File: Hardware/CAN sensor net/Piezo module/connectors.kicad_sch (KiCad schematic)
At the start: 8 parts, among them J1 532610671, J2 532610671, J3 USB_B_Micro, J4 530470310, U7 USBLC6-2SC6

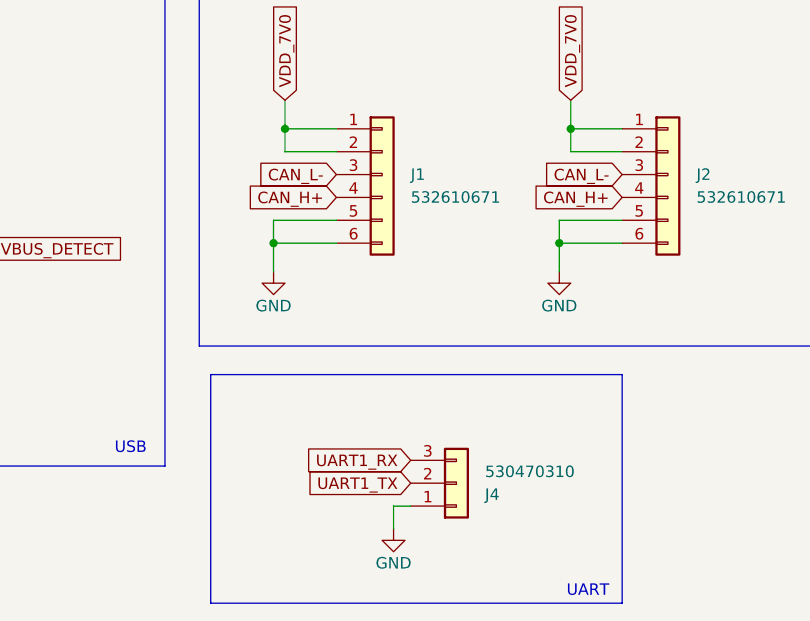
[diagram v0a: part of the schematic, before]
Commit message: Piezo concept (full)
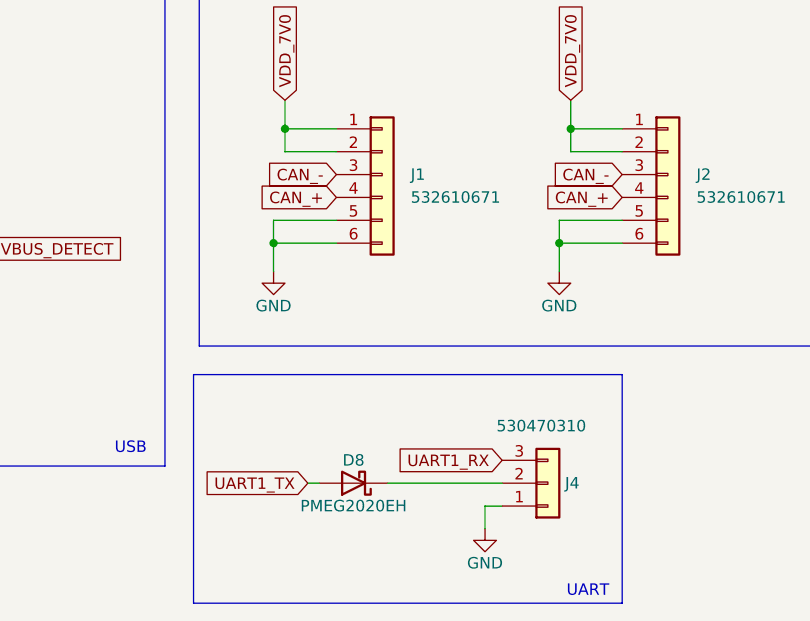
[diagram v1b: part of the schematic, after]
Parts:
- added D8: PMEG2020EH, Diode_SMD:D_SOD-123F, symbol Device:D_Schottky
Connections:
- net UART1_TX: now also D8.2 (A); no longer J4.2 (Pin_2)
- net CAN_H+ renamed CAN_+
- net CAN_L- renamed CAN_-
- new net: D8.1 (K), J4.2 (Pin_2)
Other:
- moved on the sheet: J4
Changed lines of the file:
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@@
 	(wire
 		(pts
+			(xy 174.625 79.375) (xy 175.895 79.375)
+		)
+		(stroke
+			(width 0)
+			(type default)
+		)
+	)
+	(wire
+		(pts
 			(xy 131.445 53.34) (xy 131.445 54.61)
 		)
@@
 	(wire
 		(pts
-			(xy 186.055 81.915) (xy 184.15 81.915)
+			(xy 196.215 81.915) (xy 194.31 81.915)
 		)
 		(stroke
@@
 	(wire
 		(pts
-			(xy 184.15 81.915) (xy 184.15 84.455)
+			(xy 194.31 81.915) (xy 194.31 84.455)
 		)
 		(stroke
@@
 	(wire
 		(pts
+			(xy 196.215 79.375) (xy 183.515 79.375)
+		)
+		(stroke
+			(width 0)
+			(type default)
+		)
+	)
+	(wire
+		(pts
 			(xy 97.155 64.77) (xy 97.155 66.675)
 		)
@@
 	(polyline
 		(pts
-			(xy 163.83 92.71) (xy 163.83 67.31)
+			(xy 161.925 92.71) (xy 161.925 67.31)
 		)
 		(stroke
@@
 	(polyline
 		(pts
-			(xy 163.83 92.71) (xy 209.55 92.71)
+			(xy 161.925 92.71) (xy 209.55 92.71)
 		)
 		(stroke
@@
 	(polyline
 		(pts
-			(xy 163.83 67.31) (xy 209.55 67.31)
+			(xy 161.925 67.31) (xy 209.55 67.31)
 		)
 		(stroke
@@
 		)
 	)
-	(global_label "CAN_L-"
+	(global_label "CAN_-"
 		(shape input)
 		(at 209.55 45.085 180)
@@
 		)
 		(property "Intersheetrefs" "${INTERSHEET_REFS}"
-			(at 199.3076 45.085 0)
+			(at 200.3357 45.085 0)
 			(effects
 				(font
@@
 	(global_label "UART1_TX"
 		(shape input)
-		(at 186.055 79.375 180)
+		(at 174.625 79.375 180)
 		(fields_autoplaced yes)
 		(effects
@@
 		)
 		(property "Intersheetrefs" "${INTERSHEET_REFS}"
-			(at 174.0589 79.375 0)
+			(at 162.6289 79.375 0)
 			(effects
 				(font
@@
 		)
 	)
-	(global_label "CAN_H+"
+	(global_label "CAN_+"
 		(shape input)
 		(at 209.55 47.625 180)
@@
 		)
 		(property "Intersheetrefs" "${INTERSHEET_REFS}"
-			(at 199.0052 47.625 0)
+			(at 200.3357 47.625 0)
 			(effects
 				(font
@@
 		)
 	)
-	(global_label "CAN_H+"
+	(global_label "CAN_+"
 		(shape input)
 		(at 177.8 47.625 180)
@@
 		)
 		(property "Intersheetrefs" "${INTERSHEET_REFS}"
-			(at 167.2552 47.625 0)
+			(at 168.5857 47.625 0)
 			(effects
 				(font
@@
 	(global_label "UART1_RX"
 		(shape input)
-		(at 186.055 76.835 180)
+		(at 196.215 76.835 180)
 		(fields_autoplaced yes)
 		(effects
@@
 		)
 		(property "Intersheetrefs" "${INTERSHEET_REFS}"
-			(at 173.7565 76.835 0)
+			(at 183.9165 76.835 0)
 			(effects
 				(font
@@
 		)
 	)
-	(global_label "CAN_L-"
+	(global_label "CAN_-"
 		(shape input)
 		(at 177.8 45.085 180)
@@
 		)
 		(property "Intersheetrefs" "${INTERSHEET_REFS}"
-			(at 167.5576 45.085 0)
+			(at 168.5857 45.085 0)
 			(effects
 				(font
@@
 		(pin "1"
 		)
+		(pin "MP"
+		)
 		(instances
 			(project "Piezo module"
@@
 	)
 	(symbol
+		(lib_id "Device:D_Schottky")
+		(at 179.705 79.375 180)
+		(unit 1)
+		(exclude_from_sim no)
+		(in_bom yes)
+		(on_board yes)
+		(dnp no)
+		(property "Reference" "D8"
+			(at 179.705 76.835 0)
+			(effects
+				(font
+					(size 1.27 1.27)
+				)
+			)
+		)
+		(property "Value" "PMEG2020EH"
+			(at 179.705 81.915 0)
+			(effects
+				(font
+					(size 1.27 1.27)
+				)
+			)
+		)
+		(property "Footprint" "Diode_SMD:D_SOD-123F"
+			(at 179.705 79.375 0)
+			(effects
+				(font
+					(size 1.27 1.27)
+				)
+				(hide yes)
+			)
+		)
+		(property "Datasheet" "~"
+			(at 179.705 79.375 0)
+			(effects
+				(font
+					(size 1.27 1.27)
+				)
+				(hide yes)
+			)
+		)
+		(property "Description" "Schottky diode"
+			(at 179.705 79.375 0)
+			(effects
+				(font
+					(size 1.27 1.27)
+				)
+				(hide yes)
+			)
+		)
+		(pin "2"
+		)
+		(pin "1"
+		)
+		(instances
+			(project "Piezo module"
+				(path "/0a58466e-2312-402a-82c7-7de62fe91dff/33325e08-e21c-439d-a7db-dde9f8ca3ce6"
+					(reference "D8")
+					(unit 1)
+				)
+			)
+		)
+	)
+	(symbol
 		(lib_name "GND_1")
 		(lib_id "power:GND")
@@
 		(lib_name "GND_1")
 		(lib_id "power:GND")
-		(at 184.15 84.455 0)
+		(at 194.31 84.455 0)
 		(unit 1)
 		(exclude_from_sim no)
@@
 		(dnp no)
 		(property "Reference" "#PWR018"
-			(at 184.15 90.805 0)
+			(at 194.31 90.805 0)
 			(effects
 				(font
@@
 		)
 		(property "Value" "GND"
-			(at 184.15 88.265 0)
+			(at 194.31 88.265 0)
 			(effects
 				(font
@@
 		)
 		(property "Footprint" ""
-			(at 184.15 84.455 0)
+			(at 194.31 84.455 0)
 			(effects
 				(font
@@
 		)
 		(property "Datasheet" ""
-			(at 184.15 84.455 0)
+			(at 194.31 84.455 0)
 			(effects
 				(font
@@
 		)
 		(property "Description" "Power symbol creates a global label with name \"GND\" , ground"
-			(at 184.15 84.455 0)
+			(at 194.31 84.455 0)
 			(effects
 				(font
@@
 	)
 	(symbol
+		(lib_name "Conn_01x06_1")
 		(lib_id "Connector_Generic:Conn_01x06")
 		(at 182.88 45.085 0)
@@
 		(pin "1"
 		)
+		(pin "MP"
+		)
 		(instances
 			(project "Piezo module"
@@
 	(symbol
 		(lib_id "Connector_Generic:Conn_01x03")
-		(at 191.135 79.375 0)
+		(at 201.295 79.375 0)
 		(mirror x)
 		(unit 1)
@@
 		(dnp no)
 		(property "Reference" "J4"
-			(at 194.31 80.6451 0)
+			(at 203.2 79.375 0)
 			(effects
 				(font
@@
 		)
 		(property "Value" "530470310"
-			(at 194.31 78.1051 0)
+			(at 195.58 73.025 0)
 			(effects
 				(font
@@
 		)
 		(property "Footprint" "Connector_Molex:Molex_PicoBlade_53261-0371_1x03-1MP_P1.25mm_Horizontal"
-			(at 191.135 79.375 0)
+			(at 201.295 79.375 0)
 			(effects
 				(font
@@
 		)
 		(property "Datasheet" "~"
-			(at 191.135 79.375 0)
+			(at 201.295 79.375 0)
 			(effects
 				(font
@@
 		)
 		(property "Description" "Generic connector, single row, 01x03, script generated (kicad-library-utils/schlib/autogen/connector/)"
-			(at 191.135 79.375 0)
+			(at 201.295 79.375 0)
 			(effects
 				(font
@@
 		(pin "1"
 		)
+		(pin "MP"
+		)
 		(instances

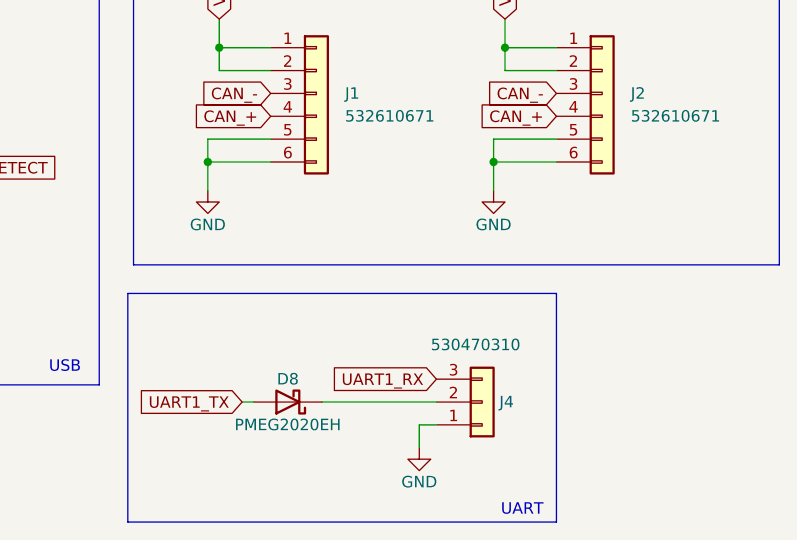
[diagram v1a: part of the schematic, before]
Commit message: Piezo production
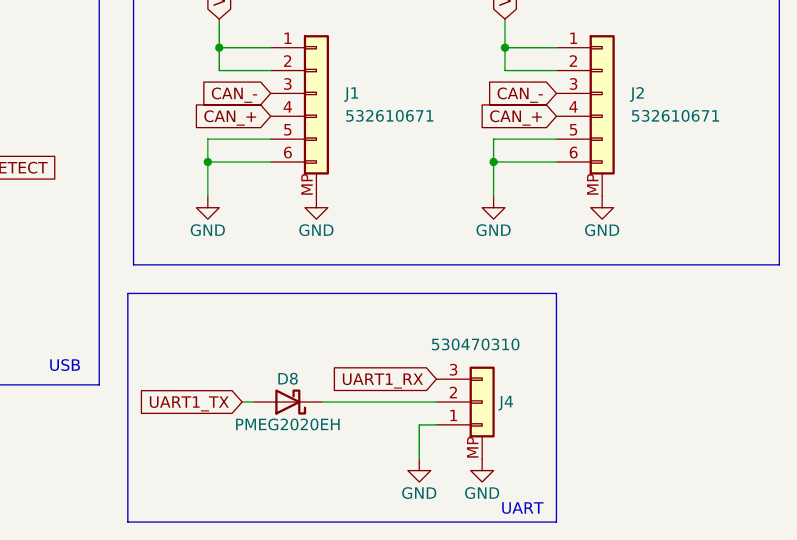
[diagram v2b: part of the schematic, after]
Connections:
- net GND: now also J1.MP, J2.MP, J4.MP
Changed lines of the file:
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@@
 	(wire
 		(pts
-			(xy 202.565 55.88) (xy 202.565 52.705)
+			(xy 202.565 56.515) (xy 202.565 52.705)
 		)
 		(stroke
@@
 	(wire
 		(pts
-			(xy 194.31 81.915) (xy 194.31 84.455)
+			(xy 194.31 81.915) (xy 194.31 85.725)
 		)
 		(stroke
@@
 	(wire
 		(pts
-			(xy 170.815 55.88) (xy 170.815 52.705)
+			(xy 170.815 56.515) (xy 170.815 52.705)
 		)
 		(stroke
@@
 	(symbol
 		(lib_id "power:GND")
+		(at 214.63 56.515 0)
+		(unit 1)
+		(exclude_from_sim no)
+		(in_bom yes)
+		(on_board yes)
+		(dnp no)
+		(property "Reference" "#PWR026"
+			(at 214.63 62.865 0)
+			(effects
+				(font
+					(size 1.27 1.27)
+				)
+				(hide yes)
+			)
+		)
+		(property "Value" "GND"
+			(at 214.63 60.325 0)
+			(effects
+				(font
+					(size 1.27 1.27)
+				)
+			)
+		)
+		(property "Footprint" ""
+			(at 214.63 56.515 0)
+			(effects
+				(font
+					(size 1.27 1.27)
+				)
+				(hide yes)
+			)
+		)
+		(property "Datasheet" ""
+			(at 214.63 56.515 0)
+			(effects
+				(font
+					(size 1.27 1.27)
+				)
+				(hide yes)
+			)
+		)
+		(property "Description" ""
+			(at 214.63 56.515 0)
+			(effects
+				(font
+					(size 1.27 1.27)
+				)
+				(hide yes)
+			)
+		)
+		(pin "1"
+		)
+		(instances
+			(project "Piezo module"
+				(path "/0a58466e-2312-402a-82c7-7de62fe91dff/33325e08-e21c-439d-a7db-dde9f8ca3ce6"
+					(reference "#PWR026")
+					(unit 1)
+				)
+			)
+		)
+	)
+	(symbol
+		(lib_id "power:GND")
 		(at 32.385 67.945 0)
 		(unit 1)
@@
 	)
 	(symbol
+		(lib_id "power:GND")
+		(at 182.88 56.515 0)
+		(unit 1)
+		(exclude_from_sim no)
+		(in_bom yes)
+		(on_board yes)
+		(dnp no)
+		(property "Reference" "#PWR025"
+			(at 182.88 62.865 0)
+			(effects
+				(font
+					(size 1.27 1.27)
+				)
+				(hide yes)
+			)
+		)
+		(property "Value" "GND"
+			(at 182.88 60.325 0)
+			(effects
+				(font
+					(size 1.27 1.27)
+				)
+			)
+		)
+		(property "Footprint" ""
+			(at 182.88 56.515 0)
+			(effects
+				(font
+					(size 1.27 1.27)
+				)
+				(hide yes)
+			)
+		)
+		(property "Datasheet" ""
+			(at 182.88 56.515 0)
+			(effects
+				(font
+					(size 1.27 1.27)
+				)
+				(hide yes)
+			)
+		)
+		(property "Description" ""
+			(at 182.88 56.515 0)
+			(effects
+				(font
+					(size 1.27 1.27)
+				)
+				(hide yes)
+			)
+		)
+		(pin "1"
+		)
+		(instances
+			(project "Piezo module"
+				(path "/0a58466e-2312-402a-82c7-7de62fe91dff/33325e08-e21c-439d-a7db-dde9f8ca3ce6"
+					(reference "#PWR025")
+					(unit 1)
+				)
+			)
+		)
+	)
+	(symbol
 		(lib_name "GND_1")
 		(lib_id "power:GND")
@@
 		(lib_name "GND_1")
 		(lib_id "power:GND")
-		(at 194.31 84.455 0)
+		(at 194.31 85.725 0)
 		(unit 1)
 		(exclude_from_sim no)
@@
 		(dnp no)
 		(property "Reference" "#PWR018"
-			(at 194.31 90.805 0)
+			(at 194.31 92.075 0)
 			(effects
 				(font
@@
 		)
 		(property "Value" "GND"
-			(at 194.31 88.265 0)
+			(at 194.31 89.535 0)
 			(effects
 				(font
@@
 		)
 		(property "Footprint" ""
-			(at 194.31 84.455 0)
+			(at 194.31 85.725 0)
 			(effects
 				(font
@@
 		)
 		(property "Datasheet" ""
-			(at 194.31 84.455 0)
+			(at 194.31 85.725 0)
 			(effects
 				(font
@@
 		)
 		(property "Description" "Power symbol creates a global label with name \"GND\" , ground"
-			(at 194.31 84.455 0)
+			(at 194.31 85.725 0)
 			(effects
 				(font
@@
 	(symbol
 		(lib_id "power:GND")
-		(at 170.815 55.88 0)
+		(at 170.815 56.515 0)
 		(unit 1)
 		(exclude_from_sim no)
@@
 		(dnp no)
 		(property "Reference" "#PWR013"
-			(at 170.815 62.23 0)
+			(at 170.815 62.865 0)
 			(effects
 				(font
@@
 		)
 		(property "Value" "GND"
-			(at 170.815 59.69 0)
+			(at 170.815 60.325 0)
 			(effects
 				(font
@@
 		)
 		(property "Footprint" ""
-			(at 170.815 55.88 0)
+			(at 170.815 56.515 0)
 			(effects
 				(font
@@
 		)
 		(property "Datasheet" ""
-			(at 170.815 55.88 0)
+			(at 170.815 56.515 0)
 			(effects
 				(font
@@
 		)
 		(property "Description" ""
-			(at 170.815 55.88 0)
+			(at 170.815 56.515 0)
 			(effects
 				(font
@@
 	(symbol
 		(lib_id "power:GND")
-		(at 202.565 55.88 0)
+		(at 202.565 56.515 0)
 		(unit 1)
 		(exclude_from_sim no)
@@
 		(dnp no)
 		(property "Reference" "#PWR014"
-			(at 202.565 62.23 0)
+			(at 202.565 62.865 0)
 			(effects
 				(font
@@
 		)
 		(property "Value" "GND"
-			(at 202.565 59.69 0)
+			(at 202.565 60.325 0)
 			(effects
 				(font
@@
 		)
 		(property "Footprint" ""
-			(at 202.565 55.88 0)
+			(at 202.565 56.515 0)
 			(effects
 				(font
@@
 		)
 		(property "Datasheet" ""
-			(at 202.565 55.88 0)
+			(at 202.565 56.515 0)
 			(effects
 				(font
@@
 		)
 		(property "Description" ""
-			(at 202.565 55.88 0)
+			(at 202.565 56.515 0)
 			(effects
 				(font
@@
 					(unit 1)
 				)
+			)
+		)
+	)
+	(symbol
+		(lib_name "GND_1")
+		(lib_id "power:GND")
+		(at 201.295 85.725 0)
+		(unit 1)
+		(exclude_from_sim no)
+		(in_bom yes)
+		(on_board yes)
+		(dnp no)
+		(property "Reference" "#PWR027"
+			(at 201.295 92.075 0)
+			(effects
+				(font
+					(size 1.27 1.27)
+				)
+				(hide yes)
+			)
+		)
+		(property "Value" "GND"
+			(at 201.295 89.535 0)
+			(effects
+				(font
+					(size 1.27 1.27)
+				)
+			)
+		)
+		(property "Footprint" ""
+			(at 201.295 85.725 0)
+			(effects
+				(font
+					(size 1.27 1.27)
+				)
+				(hide yes)
+			)
+		)
+		(property "Datasheet" ""
+			(at 201.295 85.725 0)
+			(effects
+				(font
+					(size 1.27 1.27)
+				)
+				(hide yes)
+			)
+		)
+		(property "Description" "Power symbol creates a global label with name \"GND\" , ground"
+			(at 201.295 85.725 0)
+			(effects
+				(font
+					(size 1.27 1.27)
+				)
+				(hide yes)
+			)
+		)
+		(pin "1"
+		)
+		(instances
+			(project "Piezo module"
+				(path "/0a58466e-2312-402a-82c7-7de62fe91dff/33325e08-e21c-439d-a7db-dde9f8ca3ce6"
+					(reference "#PWR027")
+					(unit 1)
+				)
